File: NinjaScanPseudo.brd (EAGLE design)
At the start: 25.4 x 35.6 mm, 59 parts, among them CON2 ZX62-B-5PA(11), CON3 JST_SH-12SM, IC1 LTC3550EDHC, IC2 MPU-6000, IC4 MAG3110FCR, J1 JUMPER1608, U1 DM3AT-SF-PEJM5, U2 H.FL, U3 NEO-6T, U4 MS5611-01BA01

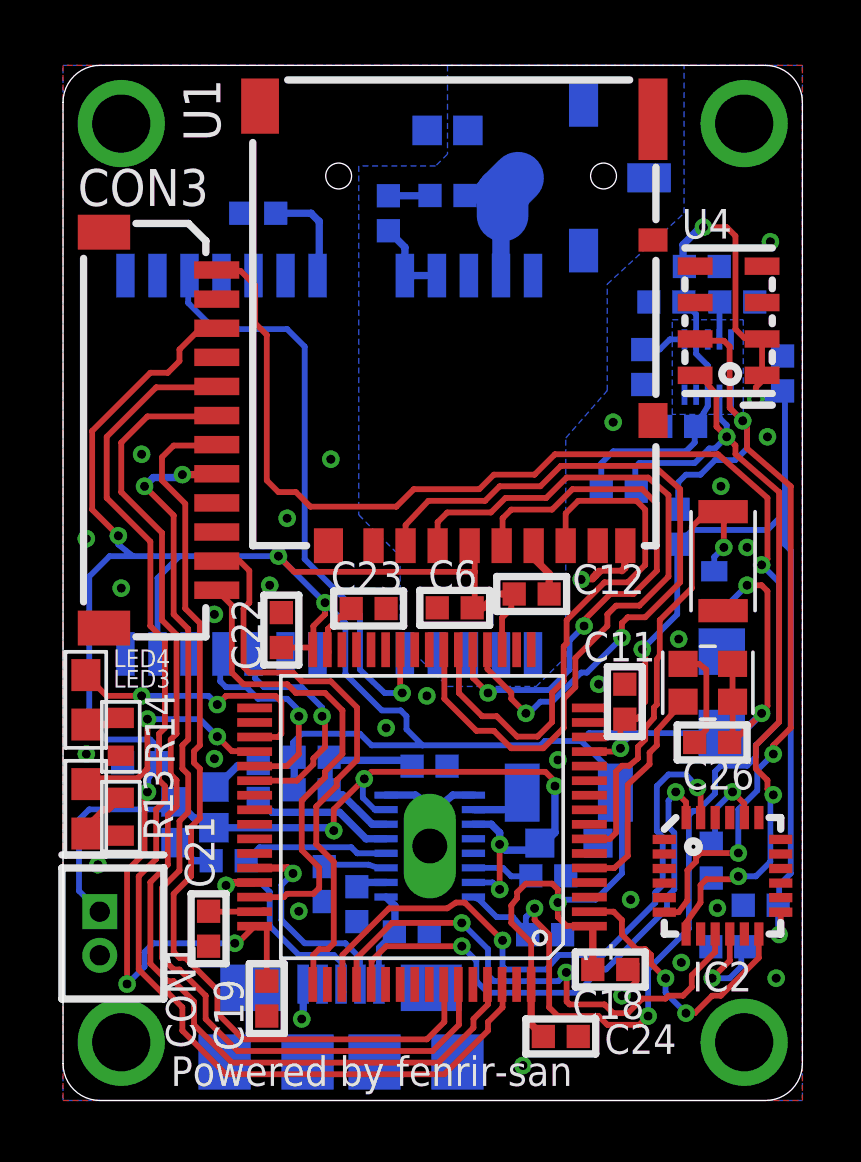
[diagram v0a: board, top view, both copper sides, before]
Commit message: Final update of Rev.A
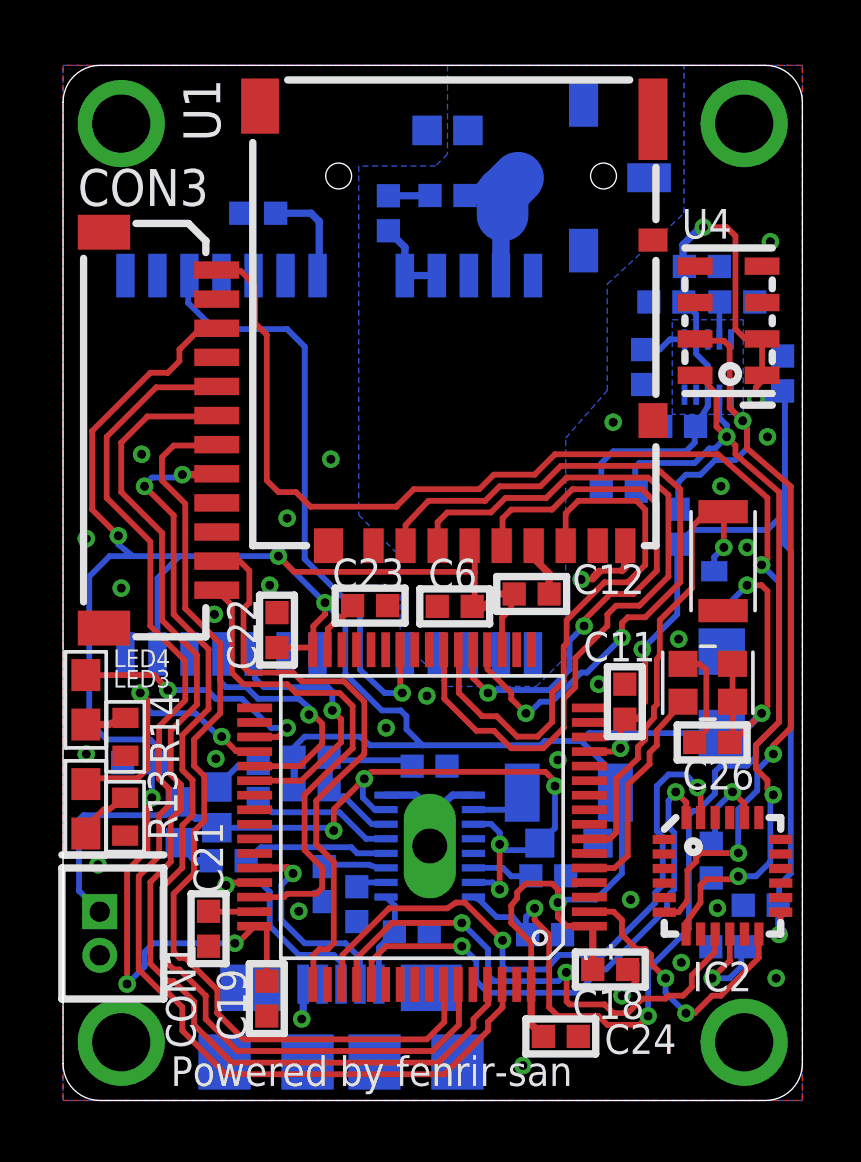
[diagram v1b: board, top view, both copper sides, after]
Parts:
- moved R14 0.16 mm to (2.14, 11.8)
- moved C22 0.15 mm to (7.35, 16.2)
- moved LED2 0.15 mm to (4.03, 9.56)
- moved R13 0.15 mm to (2.13, 9.10)
- moved C23 0.11 mm to (10.6, 17.0)
- moved LED1 0.10 mm to (5.28, 10.1)
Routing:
- net N$20: track 8.77 -> 10.6 mm
- net GPS_TX: track 7.26 -> 8.53 mm
- net GPS_RX: track 8.05 -> 9.13 mm
- net I2C1_SCL: track 39.5 -> 40.2 mm
- net USART1_TX: track 32.7 -> 33.4 mm
- net I2C1_SDA: track 40.7 -> 41.4 mm
- net USART1_RX: track 33.9 -> 34.6 mm
- net SWDIO: track 16.7 -> 17.3 mm
- net N$19: track 32.7 -> 33.3 mm
